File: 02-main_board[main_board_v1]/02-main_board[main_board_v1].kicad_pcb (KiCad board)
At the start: 4 copper layers, 91 parts, among them IC1 AD7175-8BCPZ-RL7, J1 2-84952-0, J2 2-84952-4, J3 FH41-15S-0.5SH_05_, Q1 XIAO_ESP32S3, U1 LT3973EMSE-5-PBF, U3 TPS2115ADRBR, U4 Teensy4.1, U5 PT61018PEL, U6 RCLAMP3354S_TCT, U7 ATA6561-GAQW-N, U8 74LVC4245APW_118, U9 LDL1117S50R_

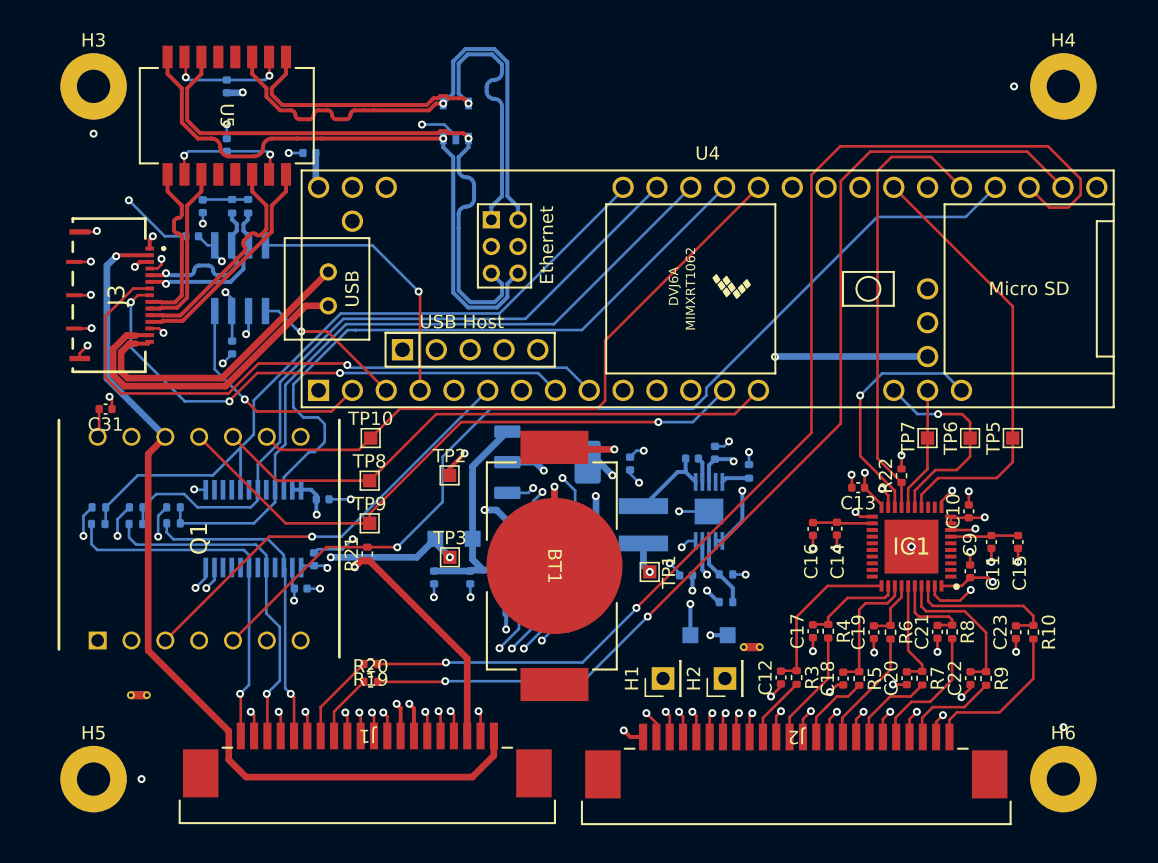
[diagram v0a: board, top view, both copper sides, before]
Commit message: first rev ready for design review
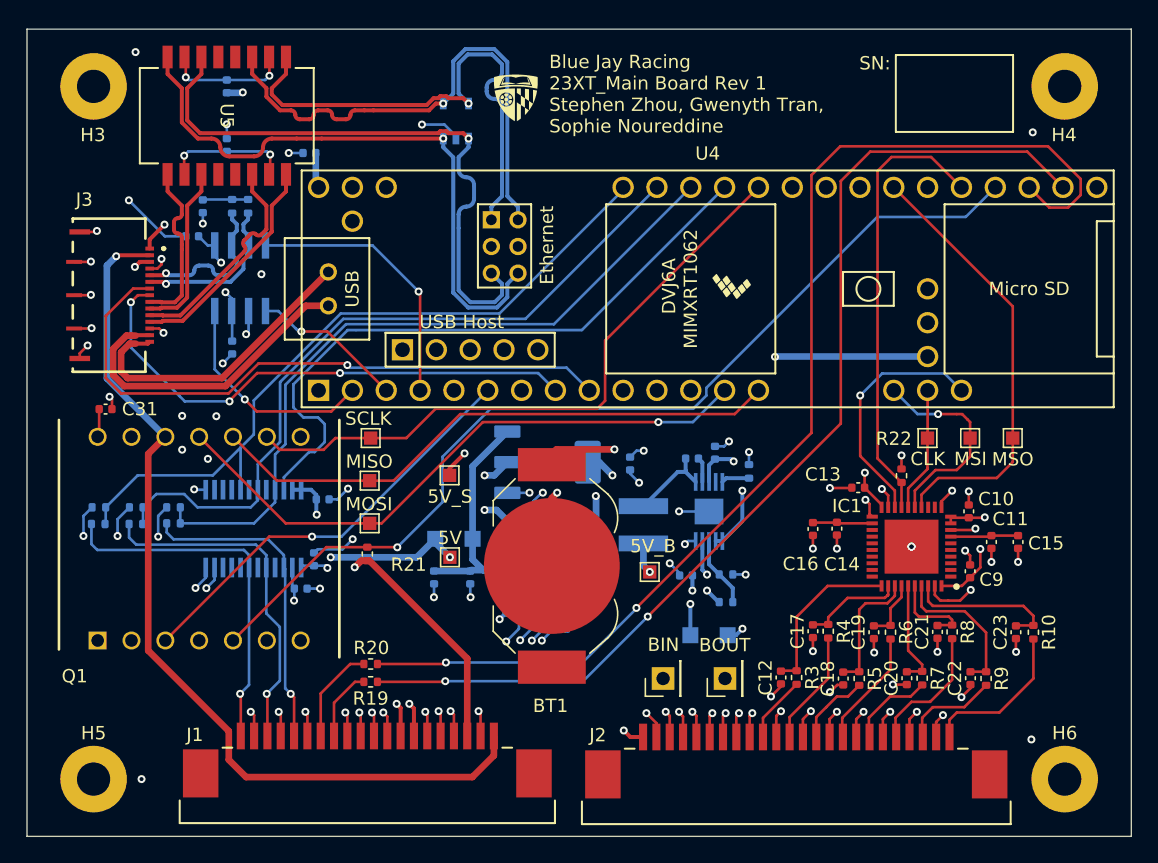
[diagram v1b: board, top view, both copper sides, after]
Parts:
- removed NT1: NetTie_1, NetTie:NetTie-2_THT_Pad0.3mm
- removed NT2: NetTie_2, NetTie:NetTie-2_THT_Pad0.3mm
- added G***: BJR_LOGO, footprints:BJR_LOGO, F.Cu at (86.9, 68.9)
- BT1: footprint footprints:BAT-HLD-012-SMT_TEC -> footprints:BatteryHolder_LINX_BAT-HLD-012-SMT
- moved H4 0.10 mm to (128.1, 68.0)
- moved H6 0.10 mm to (128.1, 120.0)
- turned BT1 to 90 degrees
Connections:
- BT1 pad 2: GNDPWR -> GNDA
- C1 pad 2: GNDPWR -> GNDA
- C13 pad 2: GNDD -> GNDA
- C14 pad 2: GNDD -> GNDA
- C16 pad 1: GNDD -> GNDA
- C24 pad 2: GNDPWR -> GNDA
- C26 pad 1: GNDPWR -> GNDA
- C27 pad 1: GNDPWR -> GNDA
- C28 pad 1: GNDPWR -> GNDA
- C29 pad 1: GNDPWR -> GNDA
- C3 pad 2: GNDPWR -> GNDA
- C30 pad 2: GNDD -> GNDA
- C31 pad 1: GNDPWR -> GNDA
- C32 pad 1: GNDPWR -> GNDA
- C33 pad 2: GNDPWR -> GNDA
- C34 pad 2: GNDPWR -> GNDA
- C4 pad 1: GNDD -> GNDA
- C6 pad 2: GNDPWR -> GNDA
- C7 pad 2: GNDPWR -> GNDA
- C8 pad 2: GNDPWR -> GNDA
- C9 pad 2: GNDD -> GNDA
- H3 pad 1: GNDPWR -> GNDA
- H5 pad 1: GNDPWR -> GNDA
- IC1 pad 19: GNDD -> GNDA
- IC1 pad 21: GNDD -> GNDA
- IC1 pad 39: GNDD -> GNDA
- IC1 pad 41: GNDD -> GNDA
- J1 pad 10: GNDD -> GNDA
- J1 pad 11: GNDD -> GNDA
- J1 pad 12: GNDD -> GNDA
- J1 pad 15: GNDD -> GNDA
- J1 pad 16: GNDD -> GNDA
- J1 pad 17: GNDD -> GNDA
- J1 pad 19: GNDD -> GNDA
- J1 pad 2: GNDD -> GNDA
- J1 pad 4: GNDD -> GNDA
- J1 pad 6: GNDD -> GNDA
- J1 pad 9: GNDD -> GNDA
- J2 pad 3: GNDPWR -> GNDA
- J2 pad 4: GNDPWR -> GNDA
- J2 pad 5: GNDPWR -> GNDA
- J3 pad 13: GNDD -> GNDA
- J3 pad 4: GNDD -> GNDA
- J3 pad G1: GNDD -> GNDA
- J3 pad G2: GNDD -> GNDA
- J3 pad G3: GNDD -> GNDA
- J3 pad MP1: GNDD -> GNDA
- J3 pad MP2: GNDD -> GNDA
- Q1 pad 13: GNDD -> GNDA
- R1 pad 2: GNDPWR -> GNDA
- R14 pad 1: GNDD -> GNDA
- R15 pad 1: GNDD -> GNDA
- R17 pad 1: GNDD -> GNDA
- R2 pad 1: GNDPWR -> GNDA
- R24 pad 1: GNDPWR -> GNDA
- U1 pad 5: GNDPWR -> GNDA
- U3 pad 2: GNDPWR -> GNDA
- U3 pad 5: GNDPWR -> GNDA
- U3 pad 9: GNDPWR -> GNDA
- U4 pad 1: GNDD -> GNDA
- U4 pad 47: GNDD -> GNDA
- U4 pad 52: GNDD -> GNDA
- U4 pad 58: GNDD -> GNDA
- U4 pad 59: GNDD -> GNDA
- U4 pad 64: GNDD -> GNDA
- U6 pad 2: GNDPWR -> GNDA
- U7 pad 2: GNDD -> GNDA
- U8 pad 11: GNDD -> GNDA
- U8 pad 12: GNDD -> GNDA
- U8 pad 13: GNDD -> GNDA
- U9 pad 1: GNDPWR -> GNDA
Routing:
- net GNDA: track 46.3 -> 175.0 mm, vias 27 -> 92
- net GNDPWR: track 77.9 -> 0.00 mm, vias 30 -> 0
- net GNDD: track 58.6 -> 0.00 mm, vias 36 -> 0
- net 5V: track 22.1 -> 29.3 mm, vias 5 -> 9
- net 3.3V_teensy: track 28.0 -> 32.1 mm, vias 5 -> 6
- net Net-(BT1-+): track 32.7 -> 33.8 mm
- net GP/Int1: track 6.75 -> 7.35 mm
- net 5V_buck: track 15.3 -> 14.8 mm
- removed copper zone on In1.Cu, net GNDD
- removed copper zone on In1.Cu, net GNDPWR
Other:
- board outline added: 82.9 x 60.6 mm
- board text added: "5V"
- board text added: "5V_B"
- board text added: "5V_S"
- board text added: "BIN"
- board text added: "BOUT"
- board text added: "Blue Jay Racing 23XT_Main Board Rev 1 Stephen Zhou, Gwenyth Tran, Sophie Noureddine"
- board text added: "CLK"
- board text added: "MISO"
- board text added: "MOSI"
- board text added: "MSI"
- board text added: "MSO"
- board text added: "SCLK"
- board text added: "SN:"
